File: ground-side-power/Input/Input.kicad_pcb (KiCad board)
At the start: 2 copper layers, 37 parts, among them J1 Battery Terminals, J2 Battery Terminals, J26 Conn_01x02_Female, J3 Battery Terminals, J4 Battery Terminals, J5 455860005, J6 455860005, J7 ATX-24, J8 Conn_01x03_Female, J9 Conn_01x03_Female, K1 AZ2150-1A-12DEF, M1 Fan_PC_Chassis, SW1 GRB234A2NABA1, U1 INA180, U2 INA180

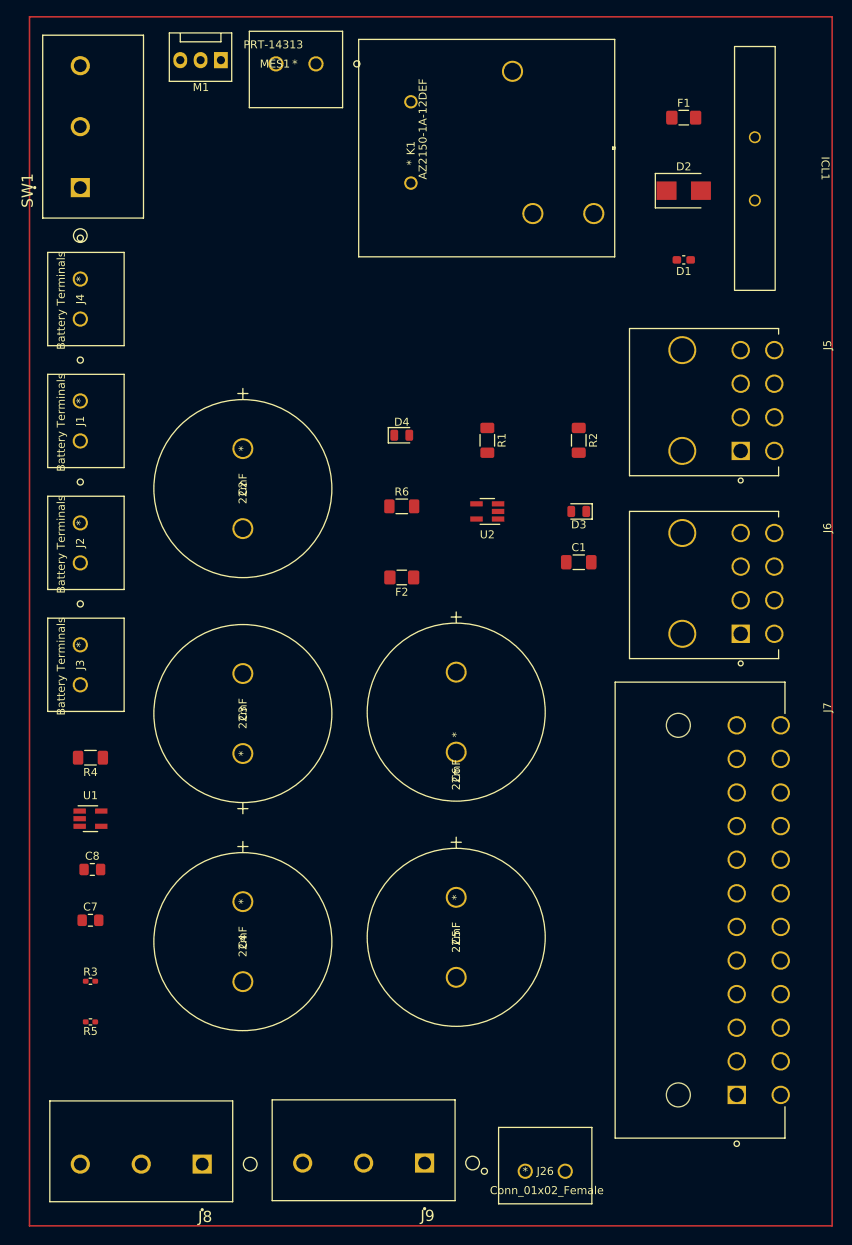
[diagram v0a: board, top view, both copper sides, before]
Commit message: PCB Layout First Draft
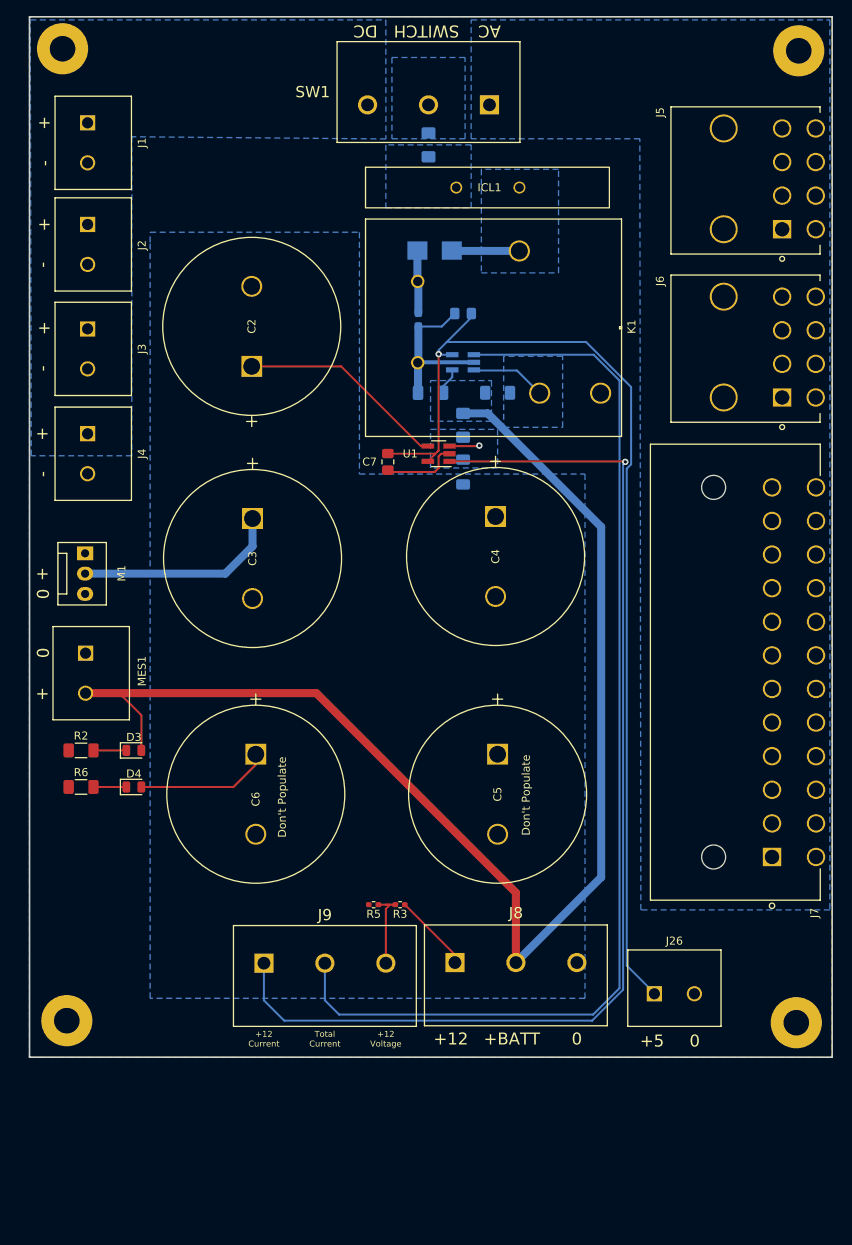
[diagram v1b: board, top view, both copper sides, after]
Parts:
- added ?: , clipboard:ee0da358-bf61-46f9-af96-80582bde7c0f, F.Cu at (44.7, 36.5)
- added ?: , , F.Cu at (45.2, 158.0)
- added ?: , , F.Cu at (136.4, 158.2)
- added ?: , , F.Cu at (136.7, 36.8)
- C1, C8, D1, D2, F1, F2, R1, R4, U2: moved to B.Cu
- K1: value AZ2150-1A-12DEF -> AZ2150_AMZ
- moved C8 83.5 mm to (94.7, 69.6)
- moved MES1 79.1 mm to (47.6, 112.1), turned to -90 degrees
- moved R2 73.3 mm to (47.0, 124.2), turned to 0 degrees
- moved C7 68.3 mm to (85.3, 88.1), turned to 90 degrees
- moved M1 63.9 mm to (47.5, 99.6), turned to -90 degrees
- moved D3 63.1 mm to (53.6, 124.2), turned to 0 degrees
- moved U1 63.1 mm to (91.7, 87.1), turned to 180 degrees
- moved R4 58.7 mm to (94.7, 89.4), turned to -90 degrees
- moved C4 57.6 mm to (98.8, 95.0)
- moved D4 55.3 mm to (53.6, 128.8)
- moved R6 53.3 mm to (47.0, 128.8)
- moved SW1 52.2 mm to (98.0, 43.5), turned to 180 degrees
- moved J8 40.4 mm to (93.7, 150.7), turned to 0 degrees
- moved R3 39.9 mm to (86.9, 143.5), turned to 180 degrees
- moved J3 39.5 mm to (47.8, 71.5)
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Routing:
- net +BATT: track 0.00 -> 166.0 mm
- net /12V_OUT: track 0.00 -> 140.3 mm, vias 0 -> 1
- net /TOTAL_OUT: track 0.00 -> 139.1 mm
- net +5V: track 0.00 -> 129.3 mm, vias 0 -> 1
- net +12V: track 0.00 -> 77.3 mm
- net GND: track 0.00 -> 30.2 mm
- net /12_VOLTAGE: track 0.00 -> 10.1 mm
- net /Sys_Sense+: track 0.00 -> 9.33 mm
- net Net-(D2-Pad2): track 0.00 -> 8.46 mm
- net Net-(D1-Pad1): track 0.00 -> 7.82 mm
- net Net-(D4-Pad1): track 0.00 -> 4.12 mm
- net Net-(D3-Pad1): track 0.00 -> 4.12 mm
- net /12V_Sense+: track 0.00 -> 3.76 mm, vias 0 -> 1
- added copper zone on B.Cu, net +12V
- added copper zone on B.Cu, net +BATT
- added copper zone on B.Cu, net /12V_Sense+
- added copper zone on B.Cu, net /ACPowerSupply
- added copper zone on B.Cu, net /BatteryPowerSupply
- added copper zone on B.Cu, net /Sys_Sense+
- added copper zone on F.Cu, net GND
- added copper zone on B.Cu, net Net-(D2-Pad2)
- added copper zone on B.Cu, net Net-(F1-Pad1)
- added copper zone on B.Cu, net Net-(F1-Pad2)
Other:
- board outline added: 100.3 x 130 mm
- board text added: "+"
- board text added: "+12"
- board text added: "+12 Current"
- board text added: "+12 Voltage"
- board text added: "+5"
- board text added: "+BATT"
- board text added: "-"
- board text added: "0"
- board text added: "AC"
- board text added: "DC"
- board text added: "Don't Populate"
- board text added: "SWITCH"
- board text added: "Total Current"
